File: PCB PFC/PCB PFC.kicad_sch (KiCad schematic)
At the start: 45 parts, among them J1 INA_1, J2 INA_2, J4 External_Power, J5 BAT54S_1, J6 BAT54S_2, SW2 SW_Push, U2 L7805, U3 TL082, U4 TL084, U5 TL082, U8 ESP32-C3_SUPERMINI_TH

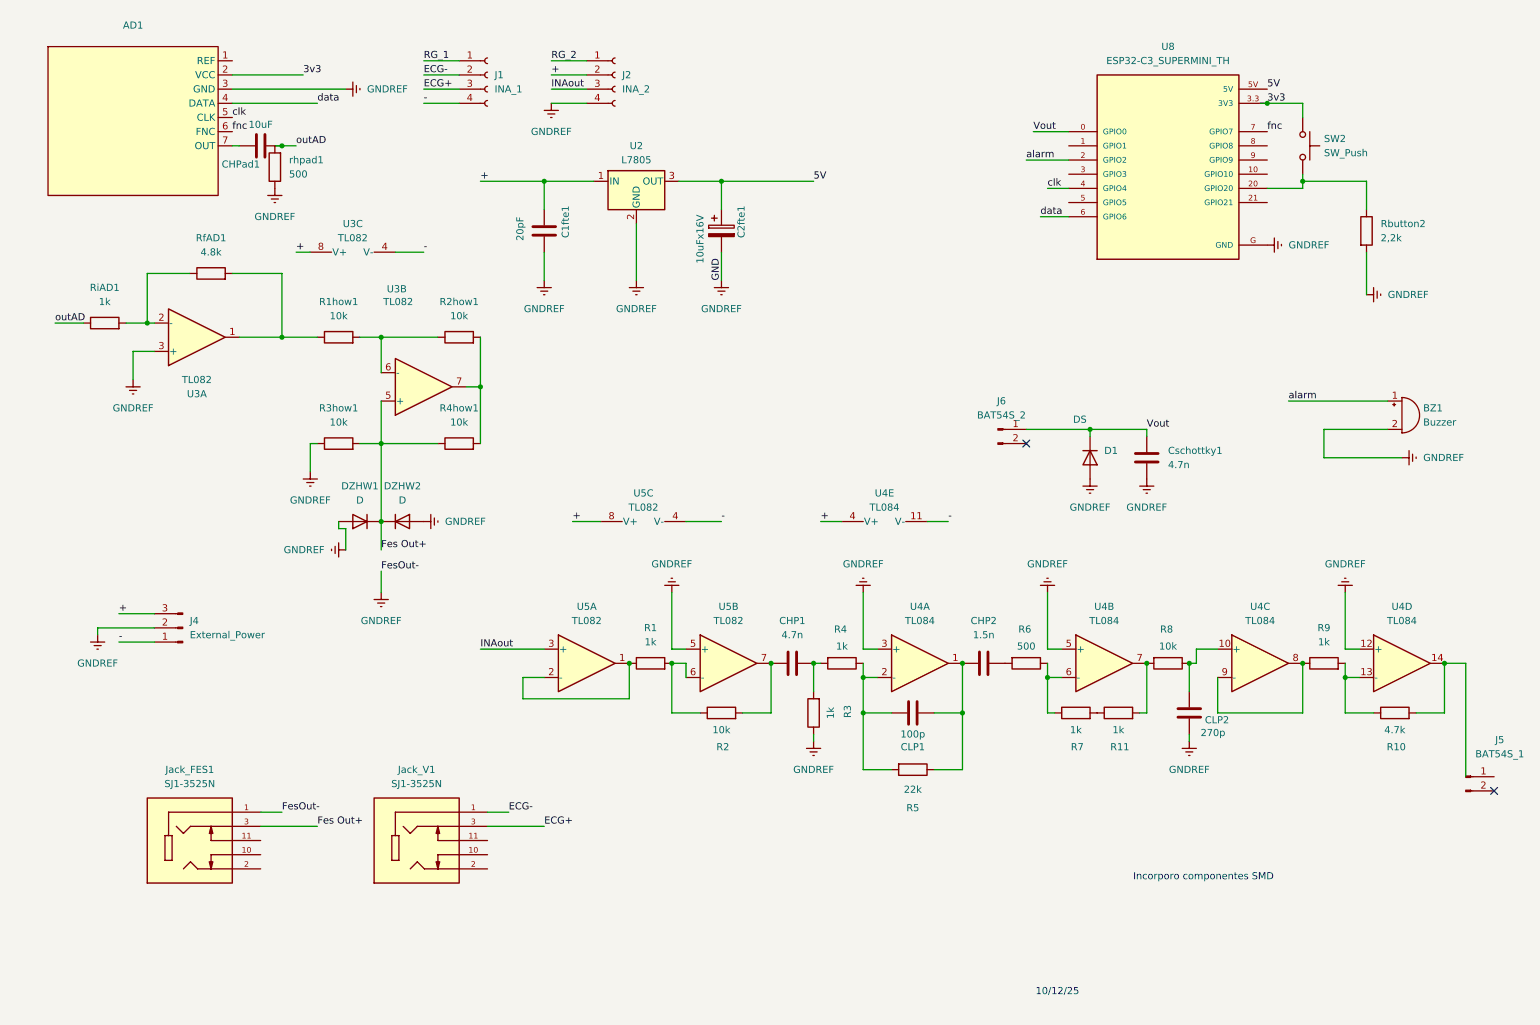
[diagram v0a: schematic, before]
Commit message: Placa final chidori 3V3 by Gus
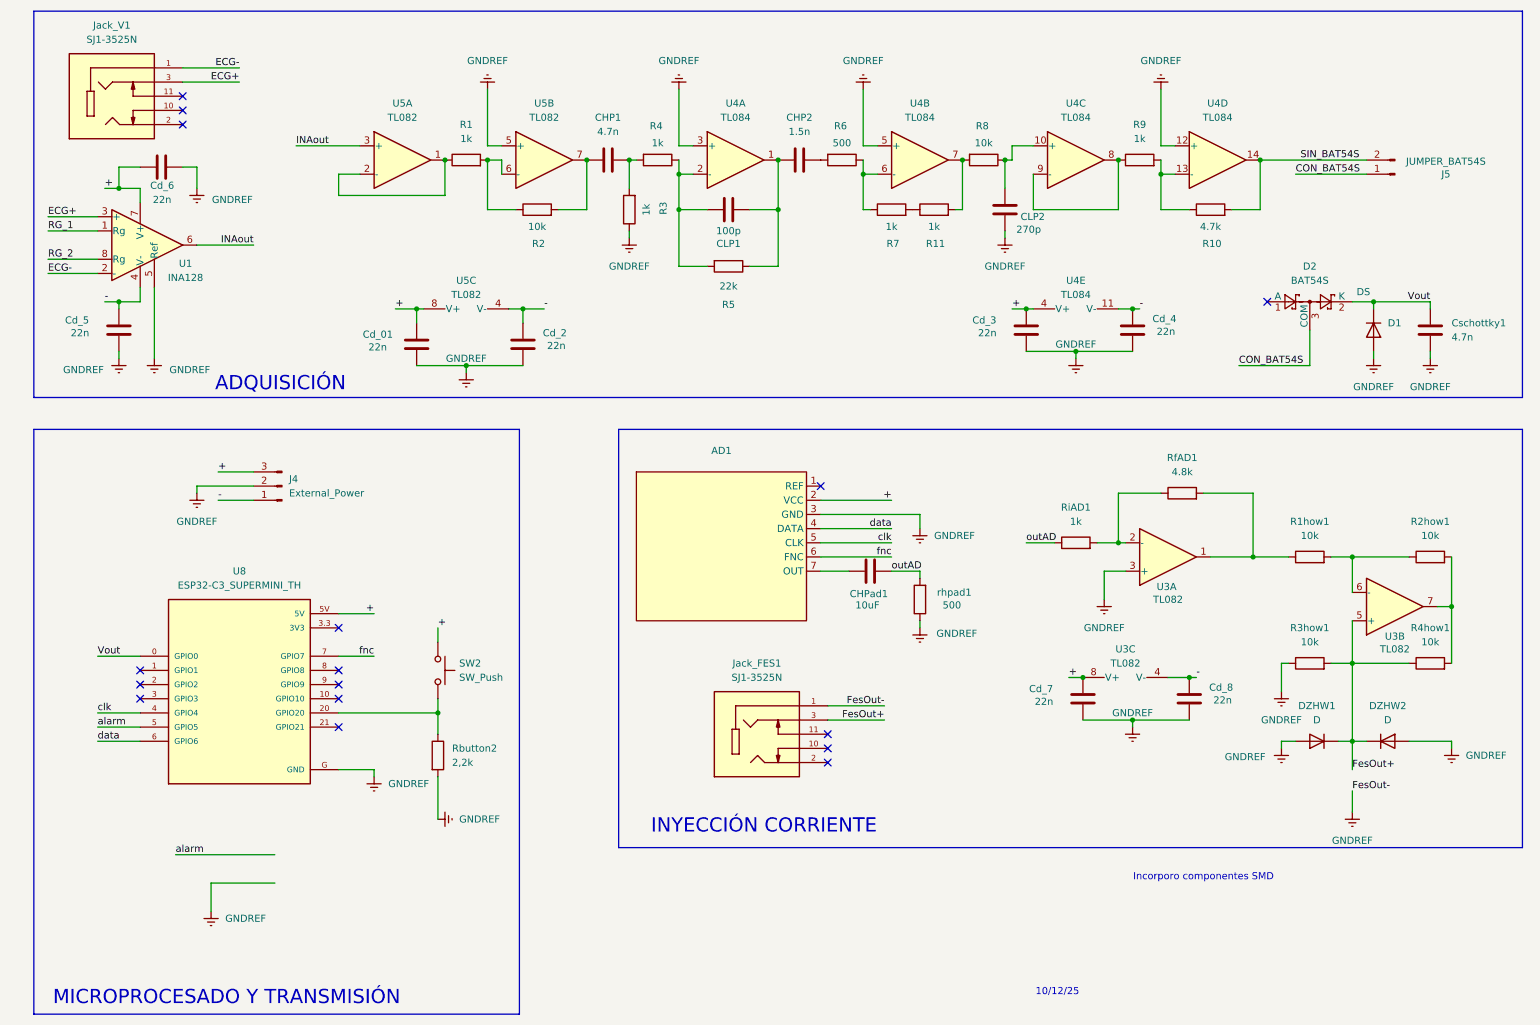
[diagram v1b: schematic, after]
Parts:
- removed BZ1: Buzzer, Buzzer_Beeper:Buzzer_12x9.5RM7.6, symbol Device:Buzzer
- removed C1fte1: 20pF, Capacitor_SMD:C_0603_1608Metric, symbol Device:C
- removed C2fte1: 10uFx16V, Capacitor_SMD:C_0805_2012Metric, symbol Device:C_Polarized
- removed J1: INA_1, Connector_PinSocket_2.54mm:PinSocket_1x04_P2.54mm_Vertical, symbol Connector:Conn_01x04_Socket
- removed J2: INA_2, Connector_PinSocket_2.54mm:PinSocket_1x04_P2.54mm_Vertical, symbol Connector:Conn_01x04_Socket
- removed J6: BAT54S_2, Connector_PinSocket_2.54mm:PinSocket_1x02_P2.54mm_Vertical, symbol Connector:Conn_01x02_Pin
- removed U2: L7805, Package_TO_SOT_THT:TO-220-3_Vertical, symbol Regulator_Linear:L7805
- added Cd_01, Cd_2, Cd_3, Cd_4, Cd_5, Cd_6, Cd_7, Cd_8: 22n, Capacitor_SMD:C_0603_1608Metric, symbol Device:C
- added D2: BAT54S, Package_TO_SOT_SMD:SOT-23, symbol Diode:BAT54S
- added U1: INA128, Package_TO_SOT_SMD:SOT-23-8, symbol Amplifier_Instrumentation:INA128
- J5: value BAT54S_1 -> JUMPER_BAT54S
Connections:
- net 5V is gone; now on net +: U8.5V
- net +: now also AD1.2 (VCC), SW2.1, Cd_01.2, Cd_3.2, Cd_6.2, Cd_7.2, U1.7 (V+)
- net -: now also Cd_2.2, Cd_4.2, Cd_5.2, Cd_8.2, U1.4 (V-)
- net ECG+: now also U1.3 (+)
- net ECG-: now also U1.2 (-)
- net GNDREF: now also Cd_01.1, Cd_2.1, Cd_3.1, Cd_4.1, Cd_5.1, Cd_6.1, Cd_7.1, Cd_8.1, U1.5 (Ref)
- net INAout: now also U1.6
- net RG_1: now also U1.1 (Rg)
- net RG_2: now also U1.8 (Rg)
- net Vout: now also D2.2 (K)
- net alarm: now also U8.5 (GPIO5); no longer U8.2 (GPIO2)
- net CON_BAT54S: now reaches J5.1 (Pin_1)
- net CON_BAT54S: now also D2.3 (COM)
- net SIN_BAT54S: now reaches J5.2 (Pin_2)
- net SIN_BAT54S: now also R10.2, U4.14
- removed net 3v3: AD1.2 (VCC), SW2.1, U8.3.3 (3V3)
- net Fes Out+ renamed FesOut+
- no-connect marks 2 -> 16
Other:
- note added: "ADQUISICIÓN"
- note added: "INYECCIÓN CORRIENTE"
- note added: "MICROPROCESADO Y TRANSMISIÓN"
- moved on the sheet: AD1, CHP1, CHP2, CHPad1, CLP1, CLP2, Cschottky1, D1, DZHW1, DZHW2, J4, J5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
